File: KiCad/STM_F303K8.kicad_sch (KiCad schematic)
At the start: 33 parts, among them IC1 TC4051BP, J10 Conn_01x02, J2 Conn_01x15_Socket, J5 Conn_01x15_Socket, J6 Conn_01x06, J9 Conn_01x02, SW2 SW_Push, SW3 SW_Push, U10 conn_02x03_pinn, U11 conn_03x03, U3 TB67H450FNG_EL, U4 TB67H450FNG_EL, U6 NJM2746M, U7 conn_03x04

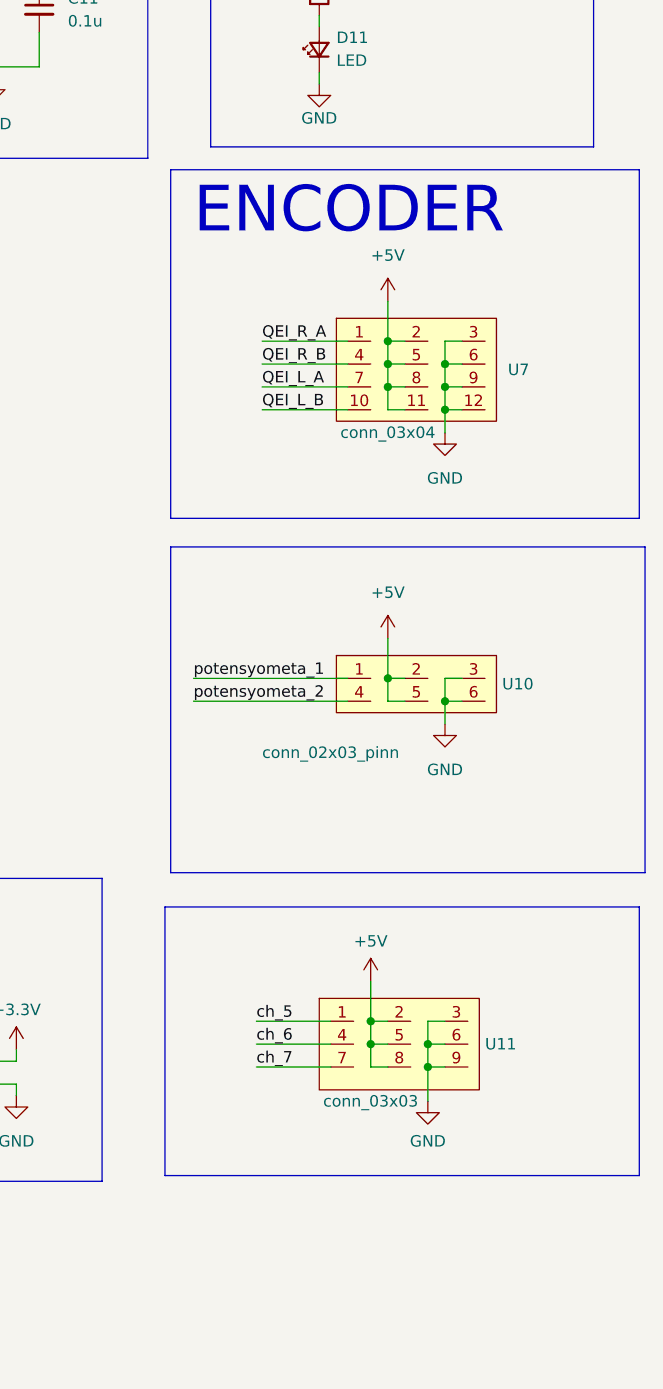
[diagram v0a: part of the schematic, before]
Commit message: I have documented the changes made.
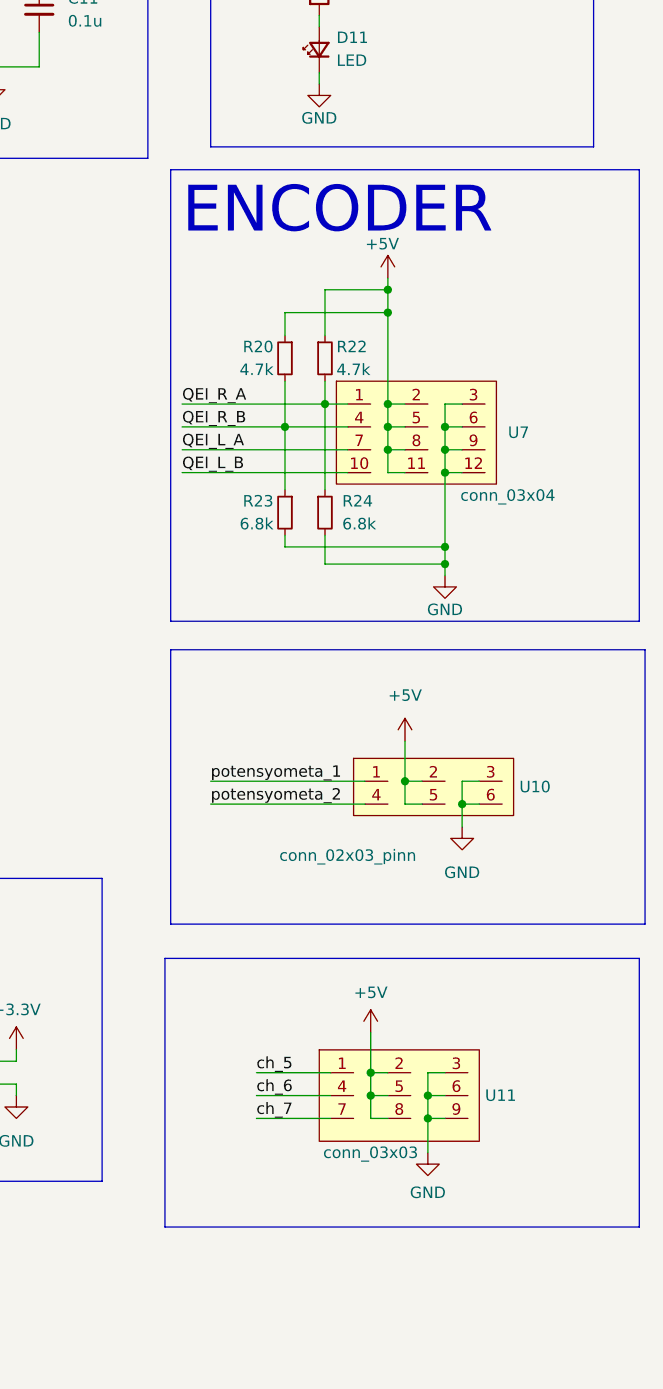
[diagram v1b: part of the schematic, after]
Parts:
- added R20, R22: 4.7k, symbol Device:R_Small
- added R23, R24: 6.8k, symbol Device:R_Small
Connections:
- net +5V: now also R20.1, R22.1
- net GND: now also R23.2, R24.2
- net QEI_R_A: now also R22.2, R24.1
- net QEI_R_B: now also R20.2, R23.1
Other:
- moved on the sheet: U10, U11, U7
